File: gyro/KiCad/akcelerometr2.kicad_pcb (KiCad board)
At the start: 2 copper layers, 24.4 x 22.4 mm, 5 parts, among them J2 Conn_01x04_Pin, J3 Conn_01x04_Pin, J4 Conn_01x08_Pin

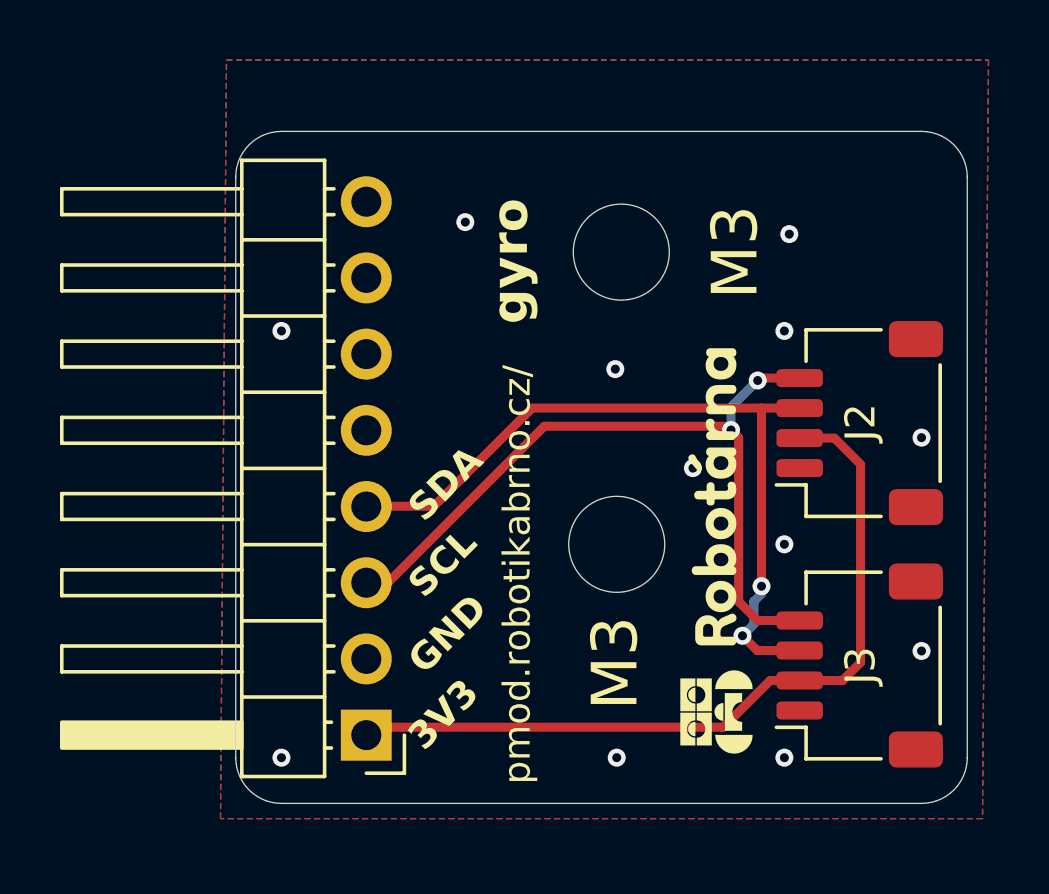
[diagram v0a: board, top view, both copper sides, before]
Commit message: Deployed d972a79 with MkDocs version: 1.6.0
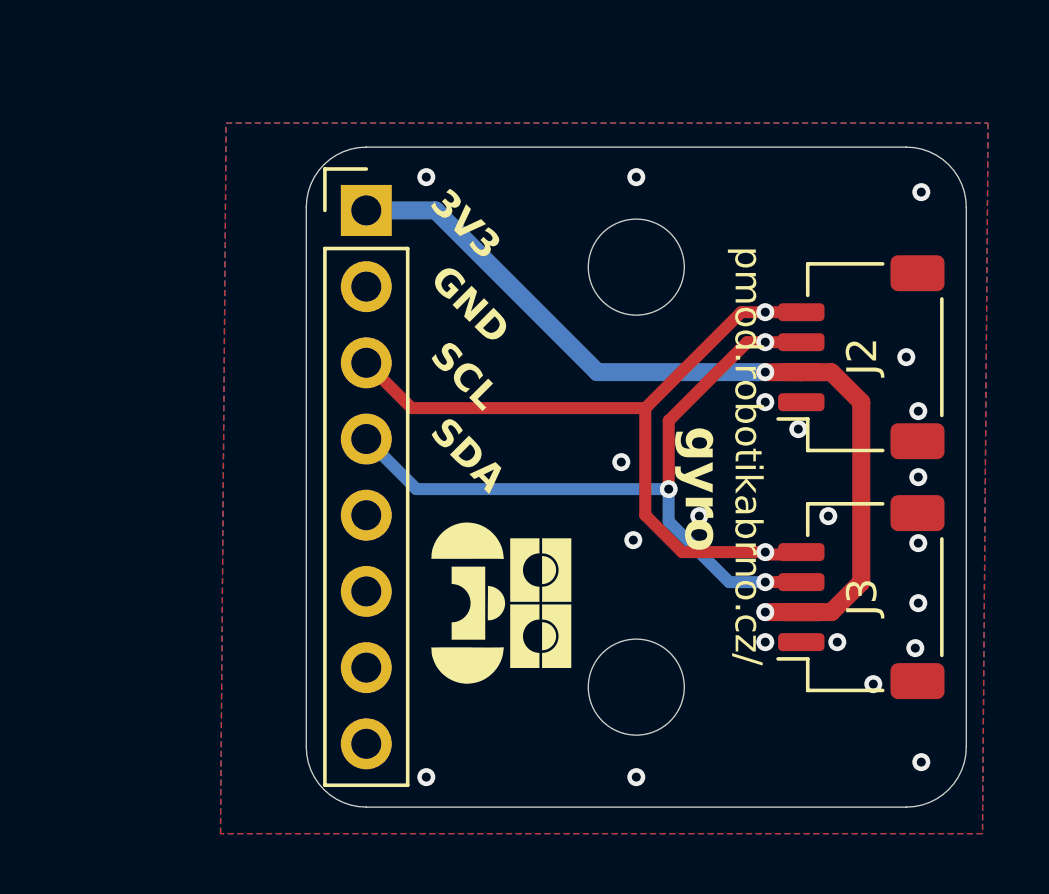
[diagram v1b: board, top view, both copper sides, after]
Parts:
- J4: value Conn_01x08_Pin -> Conn_01x06_Pin; footprint Connector_PinHeader_2.54mm:PinHeader_1x08_P2.54mm_Horizontal -> Connector_PinHeader_2.54mm:PinHeader_1x08_P2.54mm_Vertical
- moved J4 17.5 mm to (109.0, 67.6), turned to 0 degrees
- moved H2 4.80 mm to (118.0, 83.5)
- moved J3 2.28 mm to (125.5, 80.5)
- moved J2 2.20 mm to (125.5, 72.5)
- moved H1 0.71 mm to (118.0, 69.5)
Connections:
- J2 pad MP: (no net) -> GND
- J3 pad MP: (no net) -> GND
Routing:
- net +3V3: track 26.5 -> 28.8 mm, vias 0 -> 2
- net SDA: track 25.7 -> 24.8 mm, vias 2 -> 3
- net GND: vias 12 -> 21
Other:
- board size 24.4 x 22.4 mm -> 22 x 22 mm
- board text added: "20mm"
- board text added: "24mm"
- board text removed: "H2"
- board text removed: "M3"
